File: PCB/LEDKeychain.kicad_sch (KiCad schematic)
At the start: 5 parts, among them U1 13.56MHz

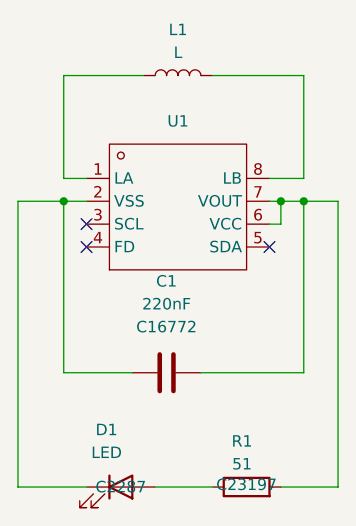
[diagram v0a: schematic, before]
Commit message: Add files via upload
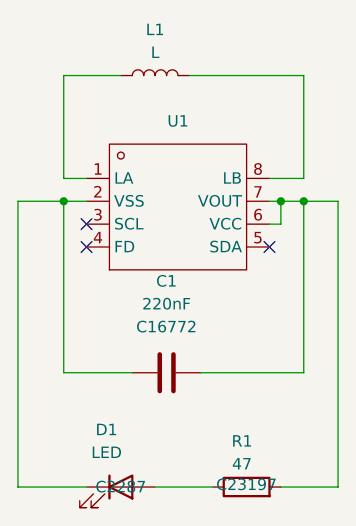
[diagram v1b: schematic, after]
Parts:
- L1: footprint Antenna:Antenna_10x7mm -> Antenna:Antenna_8500000x5500000mm
- R1: value 51 -> 47
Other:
- moved on the sheet: L1
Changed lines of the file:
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@@
 	(wire
 		(pts
-			(xy 82.55 57.15) (xy 73.66 57.15)
-		)
-		(stroke
-			(width 0)
-			(type default)
-		)
-	)
-	(wire
-		(pts
-			(xy 90.17 57.15) (xy 100.33 57.15)
+			(xy 80.01 57.15) (xy 73.66 57.15)
 		)
 		(stroke
@@
 		(pts
 			(xy 96.52 71.12) (xy 97.79 71.12)
+		)
+		(stroke
+			(width 0)
+			(type default)
+		)
+	)
+	(wire
+		(pts
+			(xy 87.63 57.15) (xy 100.33 57.15)
 		)
 		(stroke
@@
 	(symbol
 		(lib_id "Device:L")
-		(at 86.36 57.15 90)
+		(at 83.82 57.15 90)
 		(unit 1)
 		(exclude_from_sim no)
@@
 		(fields_autoplaced yes)
 		(property "Reference" "L1"
-			(at 86.36 52.07 90)
+			(at 83.82 52.07 90)
 			(effects
 				(font
@@
 		)
 		(property "Value" "L"
-			(at 86.36 54.61 90)
-			(effects
-				(font
-					(size 1.27 1.27)
-				)
-			)
-		)
-		(property "Footprint" "Antenna:Antenna_10x7mm"
-			(at 86.36 57.15 0)
+			(at 83.82 54.61 90)
+			(effects
+				(font
+					(size 1.27 1.27)
+				)
+			)
+		)
+		(property "Footprint" "Antenna:Antenna_8500000x5500000mm"
+			(at 83.82 57.15 0)
 			(effects
 				(font
@@
 		)
 		(property "Datasheet" "~"
-			(at 86.36 57.15 0)
+			(at 83.82 57.15 0)
 			(effects
 				(font
@@
 		)
 		(property "Description" "Inductor"
-			(at 86.36 57.15 0)
+			(at 83.82 57.15 0)
 			(effects
 				(font
@@
 			)
 		)
-		(property "Value" "51"
+		(property "Value" "47"
 			(at 93.472 100.33 90)
 			(effects
